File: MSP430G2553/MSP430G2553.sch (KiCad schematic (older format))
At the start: 29 parts, among them J1 Power, J2 Programmer, J3 Conn_01x06_Female, J4 Conn_01x08_Female, SW1 SW_Push, U1 MSP430G2553IPW20, Y1 Crystal_GND24

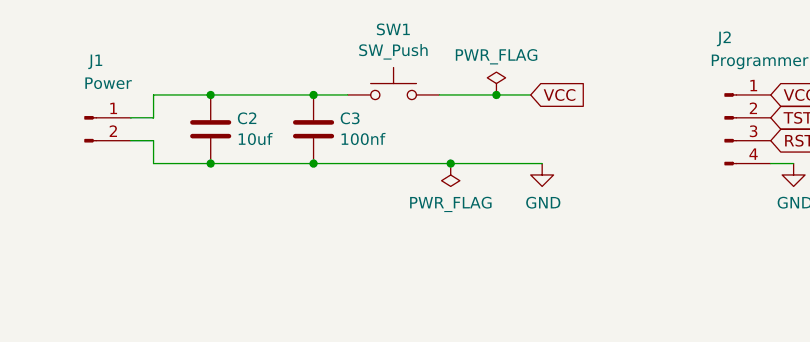
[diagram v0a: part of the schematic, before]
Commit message: Adjusted g2553.
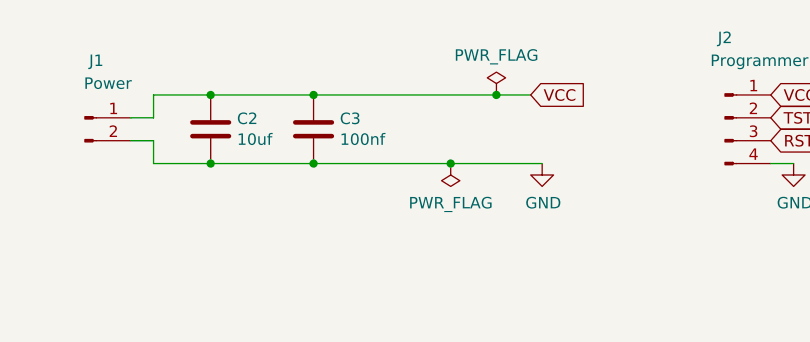
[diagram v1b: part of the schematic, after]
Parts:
- removed SW1: SW_Push, Button_Switch_SMD:SW_Push_1P1T_NO_6x6mm_H9.5mm, symbol Switch:SW_Push
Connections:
- net VCC: now also C2.1, C3.1, J1.1 (Pin_1)
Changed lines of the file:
@@
 Wire Wire Line
 	5700 2000 5800 2000
-$Comp
-L Switch:SW_Push SW1
-U 1 1 5EC1A6E2
-P 4050 1700
-F 0 "SW1" H 4050 1985 50  0000 C CNN
-F 1 "SW_Push" H 4050 1894 50  0000 C CNN
-F 2 "Button_Switch_SMD:SW_Push_1P1T_NO_6x6mm_H9.5mm" H 4050 1900 50  0001 C CNN
-F 3 "~" H 4050 1900 50  0001 C CNN
-	1    4050 1700
-	1    0    0    -1
-$EndComp
-Wire Wire Line
-	3850 1700 3700 1700
 Connection ~ 3700 1700
 Wire Wire Line
@@
 	1    0    0    -1
 $EndComp
-Wire Wire Line
-	4250 1700 4500 1700
 Wire Wire Line
 	3000 1700 3250 1700
@@
 	0    1    1    0
 $EndComp
+Wire Wire Line
+	3700 1700 4500 1700
 $EndSCHEMATC
